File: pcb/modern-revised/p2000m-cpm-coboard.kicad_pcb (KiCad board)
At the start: 2 copper layers, 88.9 x 55.6 mm, 18 parts, among them J1 CPU BOARD, J2 EXPANSION BOARD, J3 T/~{M}, J4 Atmel-JTAG-10, J5 TERMINAL, U2 CY62128, U3 DIL16, U4 ATF1502AS

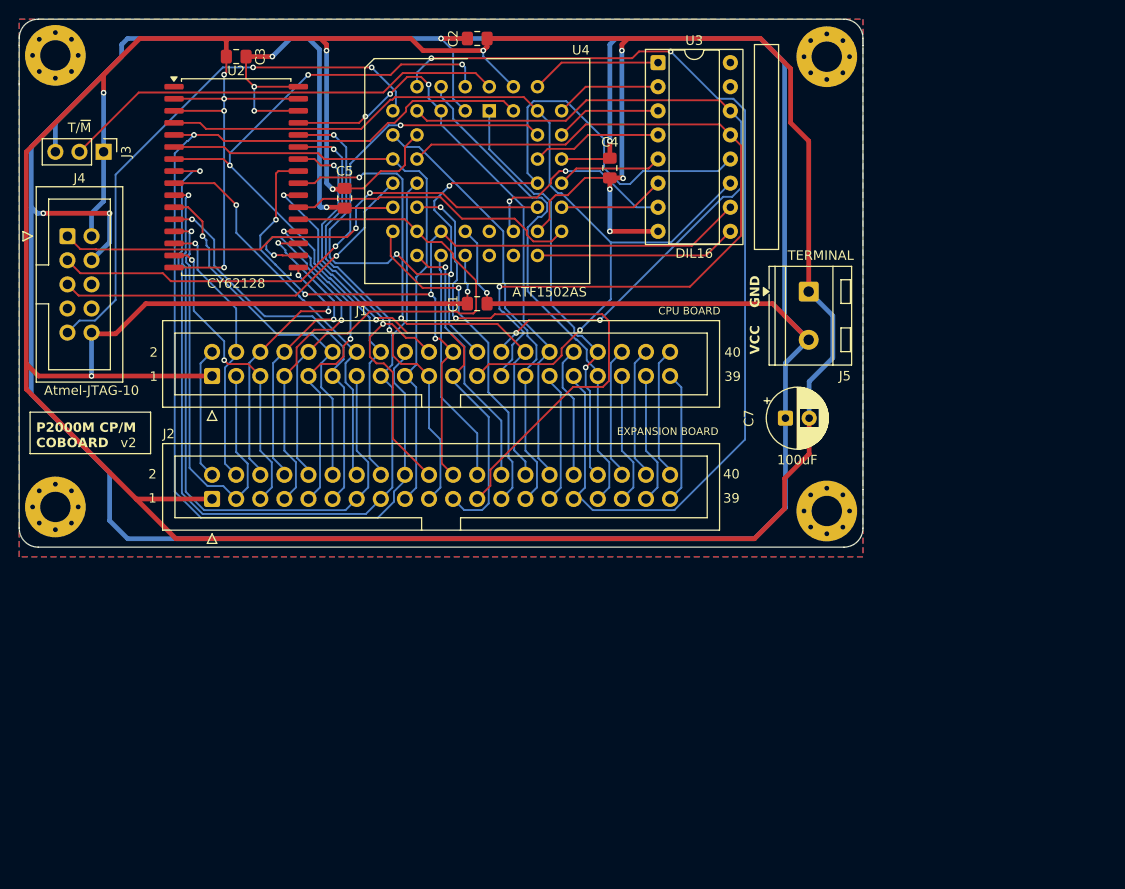
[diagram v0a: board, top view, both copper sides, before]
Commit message: Redesigning modern board
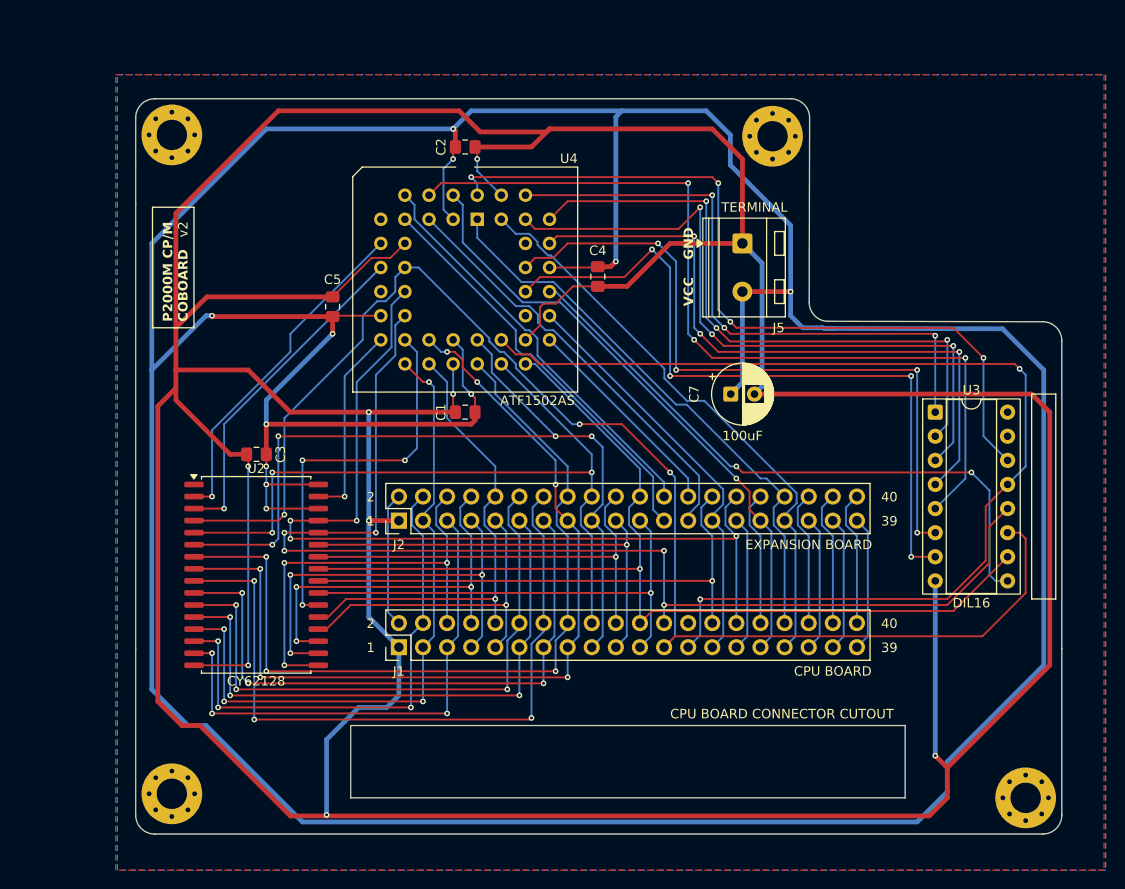
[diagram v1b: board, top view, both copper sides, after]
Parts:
- removed J3: T/~{M}, Connector_PinHeader_2.54mm:PinHeader_1x03_P2.54mm_Vertical
- removed J4: Atmel-JTAG-10, Connector_IDC:IDC-Header_2x05_P2.54mm_Vertical
- J1, J2: footprint Connector_IDC:IDC-Header_2x20_P2.54mm_Vertical -> Connector_PinHeader_2.54mm:PinHeader_2x20_P2.54mm_Vertical
- moved U3 47.0 mm to (111.8, 58.4)
- moved C3 42.0 mm to (40.2, 62.9)
- moved U2 42.0 mm to (40.2, 75.6)
- moved H4 36.8 mm to (121.3, 99.1)
- moved J1 34.7 mm to (55.2, 83.2)
- moved H2 32.6 mm to (31.3, 98.6)
- moved J2 19.8 mm to (55.2, 69.8)
- moved H1 14.9 mm to (31.3, 29.2)
- moved C1 11.5 mm to (62.2, 58.4)
- moved C2 11.5 mm to (62.2, 30.5)
- moved C4 11.5 mm to (76.2, 44.1)
- moved C5 11.5 mm to (48.3, 47.3)
- moved U4 11.5 mm to (63.5, 38.1)
- moved H3 10.1 mm to (94.6, 29.4)
- moved J5 8.63 mm to (91.4, 40.6)
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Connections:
- J1 pad 26: A15 -> unconnected-(J1-Pin_26-Pad26)
- J2 pad 26: RA15 -> RAMS2_EXP
- U2 pad 2: GND -> A16_RAM
- U2 pad 3: GND -> A14_RAM
- U2 pad 31: GND -> A15_RAM
- U4 pad 11: A6 -> A14_RAM
- U4 pad 12: A14 -> A12
- U4 pad 13: TMS -> unconnected-(U4-I/O/TMS-Pad13)
- U4 pad 14: A4 -> ~{WR}
- U4 pad 16: RA12 -> A13
- U4 pad 17: RA14 -> A15_RAM
- U4 pad 18: RA15 -> D0
- U4 pad 19: D7 -> ~{RAMS3}
- U4 pad 2: A5 -> ~{IORQ}
- U4 pad 20: RA13 -> D7
- U4 pad 21: A11 -> A4
- U4 pad 24: unconnected-(U4-I/O-Pad24) -> A5
- U4 pad 25: unconnected-(U4-I/O/PD2-Pad25) -> A6
- U4 pad 26: unconnected-(U4-I/O-Pad26) -> A7
- U4 pad 27: P6 -> A14
- U4 pad 28: P7 -> A11
- U4 pad 29: ~{RAMS3} -> RAMS2_EXP
- U4 pad 31: P5 -> ~{MRQ}
- U4 pad 32: TCK -> unconnected-(U4-I/O/TCK-Pad32)
- U4 pad 33: P4 -> P7
- U4 pad 34: A13 -> P6
- U4 pad 36: P3 -> P5
- U4 pad 37: P2 -> P3
- U4 pad 38: TDO -> unconnected-(U4-I/O/TDO-Pad38)
- U4 pad 4: ~{M1} -> P4
- U4 pad 41: A12 -> P2
- U4 pad 43: A7 -> ~{M1}
- U4 pad 44: Net-(J3-Pin_2) -> A15
- U4 pad 5: ~{WR} -> RA14
- U4 pad 6: ~{IORQ} -> RA13
- U4 pad 7: TDI -> unconnected-(U4-I/O/TDI-Pad7)
- U4 pad 8: A15 -> RA12
- U4 pad 9: ~{MRQ} -> A16_RAM
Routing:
- net P4: track 11.2 -> 91.2 mm, vias 0 -> 3
- net P5: track 11.2 -> 73.6 mm, vias 0 -> 4
- net TDO: track 61.8 -> 0.00 mm, vias 2 -> 0
- net P2: track 11.2 -> 72.5 mm, vias 0 -> 3
- net GND: track 468.3 -> 529.1 mm, vias 14 -> 8
- net VCC: track 388.6 -> 447.6 mm, vias 9 -> 11
- net TDI: track 57.1 -> 0.00 mm, vias 2 -> 0
- net P1: track 11.2 -> 66.8 mm, vias 0 -> 3
- net P3: track 13.8 -> 69.2 mm, vias 0 -> 3
- net TCK: track 54.5 -> 0.00 mm, vias 2 -> 0
- net P6: track 22.1 -> 76.3 mm, vias 2 -> 4
- net P0: track 13.8 -> 64.8 mm, vias 0 -> 3
- net A12: track 96.9 -> 146.4 mm, vias 1 -> 3
- net Net-(J3-Pin_2): track 47.2 -> 0.00 mm
- net ~{IORQ}: track 109.5 -> 64.3 mm, vias 2 -> 1
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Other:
- board size 88.9 x 55.6 mm -> 97.6 x 77.5 mm
- board text added: "CPU BOARD CONNECTOR CUTOUT"
